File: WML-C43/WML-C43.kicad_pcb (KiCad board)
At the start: 2 copper layers, 14 parts, among them J1 TYPE-C-31-M12_13, U1 USBLC6-2SC6, U2 MCP1700-3302E_SOT23, U3 WML-C43

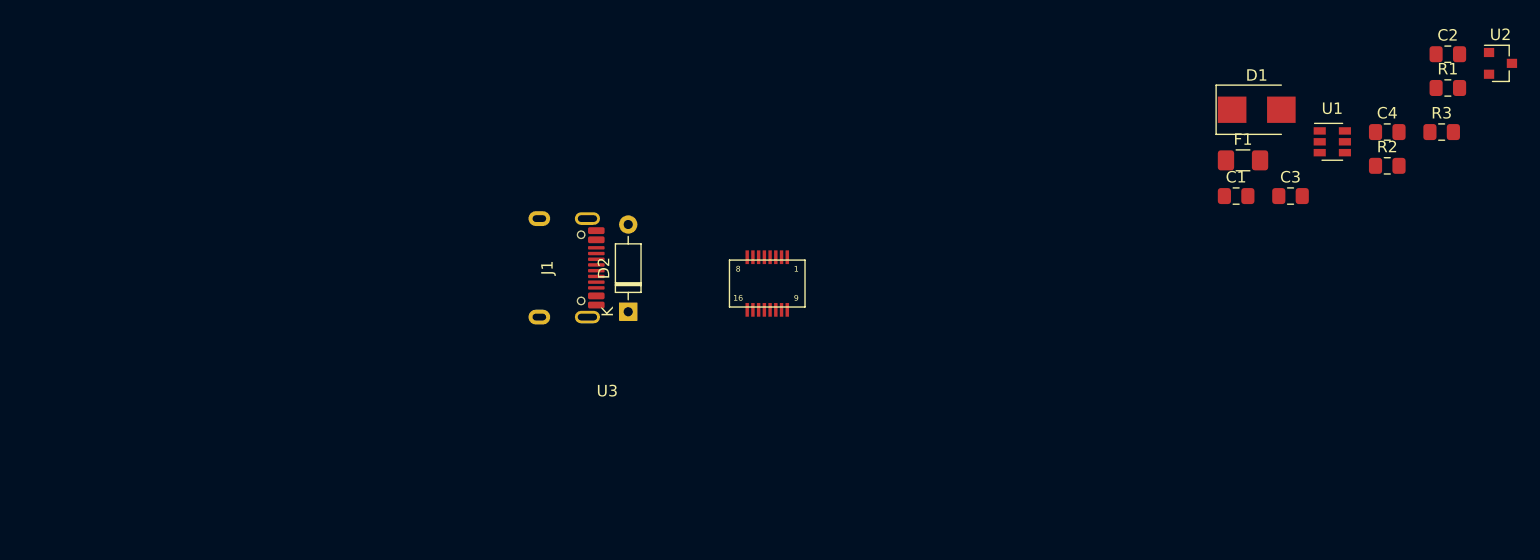
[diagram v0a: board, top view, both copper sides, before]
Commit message: pcb finish i think
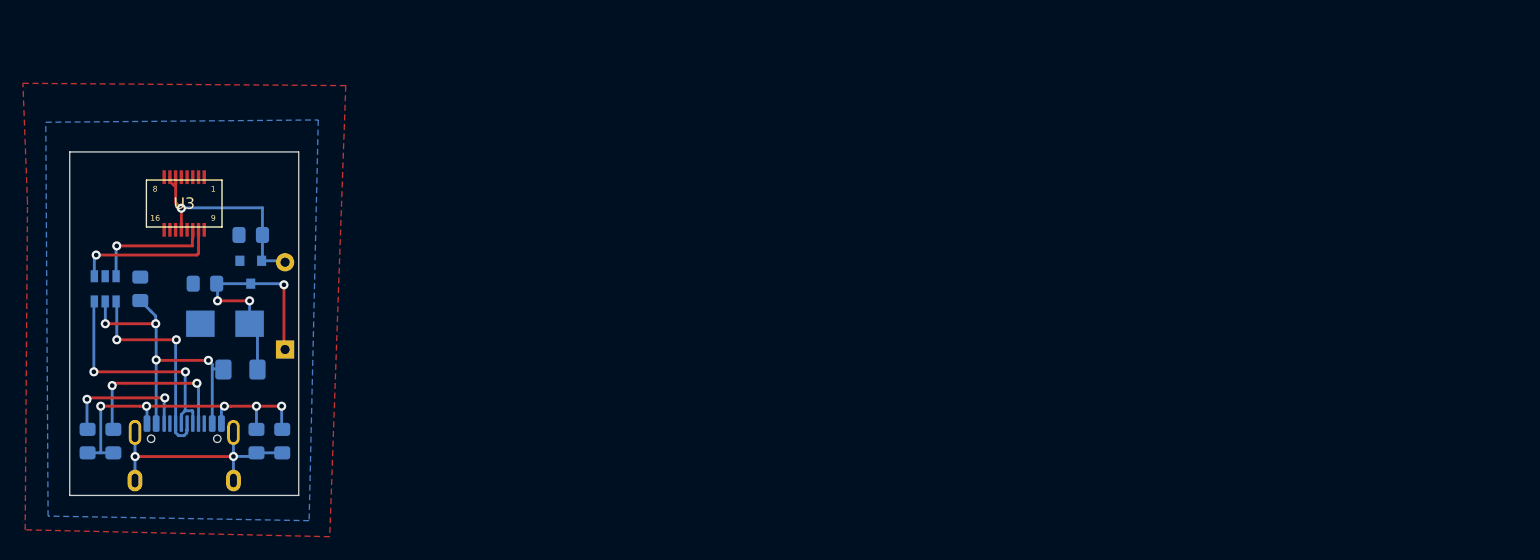
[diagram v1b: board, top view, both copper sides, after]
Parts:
- C1, C2, C3, C4, D1, D2, F1, J1, R1, R2, R3, U1, U2: moved to B.Cu
- moved R3 121.3 mm to (151.6, 55.3), turned to 270 degrees
- moved R2 113.8 mm to (153.8, 55.3), turned to 270 degrees
- moved U2 110.7 mm to (165.8, 40.5), turned to 270 degrees
- moved C2 110.4 mm to (161.8, 41.5), turned to 180 degrees
- moved U1 107.9 mm to (153.1, 42.0), turned to 270 degrees
- moved R1 106.4 mm to (168.6, 55.3), turned to 90 degrees
- moved C3 100.8 mm to (156.2, 42.0), turned to 270 degrees
- moved C4 99.7 mm to (165.8, 37.3), turned to 180 degrees
- moved D1 92.0 mm to (163.6, 45.0), turned to 180 degrees
- moved F1 89.5 mm to (164.9, 49.0), turned to 180 degrees
- moved C1 88.2 mm to (166.3, 55.3), turned to 90 degrees
- moved U3 51.4 mm to (160.0, 34.5)
- moved J1 38.9 mm to (160.0, 53.0), turned to 180 degrees
- moved D2 30.2 mm to (168.8, 47.3)
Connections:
- U3 pad 1: (no net) -> GND
- U3 pad 10: (no net) -> D-
- U3 pad 11: (no net) -> D+
- U3 pad 13: (no net) -> 3.3V
- U3 pad 16: (no net) -> GND
- U3 pad 6: (no net) -> 3.3V
- U3 pad 7: (no net) -> 3.3V
- U3 pad 8: (no net) -> GND
- U3 pad 9: (no net) -> GND
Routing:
- net VBUS: track 0.00 -> 31.2 mm, vias 0 -> 4
- net GND: track 0.00 -> 30.5 mm, vias 0 -> 5
- net Net-(C2-Pad1): track 0.00 -> 23.5 mm, vias 0 -> 3
- net DBUS-: track 0.00 -> 21.7 mm, vias 0 -> 2
- net Net-(C1-Pad1): track 0.00 -> 21.4 mm, vias 0 -> 2
- net 3.3V: track 0.00 -> 19.7 mm, vias 0 -> 1
- net DBUS+: track 0.00 -> 18.2 mm, vias 0 -> 2
- net Net-(J1-PadA5): track 0.00 -> 15.5 mm, vias 0 -> 2
- net D-: track 0.00 -> 13.0 mm, vias 0 -> 1
- net Net-(J1-PadB5): track 0.00 -> 12.3 mm, vias 0 -> 2
- net D+: track 0.00 -> 10.7 mm, vias 0 -> 1
- added copper zone on B.Cu, net GND
- added copper zone on F.Cu, net GND
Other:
- board outline added: 20 x 30 mm
